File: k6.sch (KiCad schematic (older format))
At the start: 23 parts, among them J1 USB_C_Receptacle_USB2.0, J2 Conn_02x05_Odd_Even, SW1 SW_SPDT, SW2 SW_Push, U1 STM32F042K6T6, U2 MCP1700-3302E_SOT23

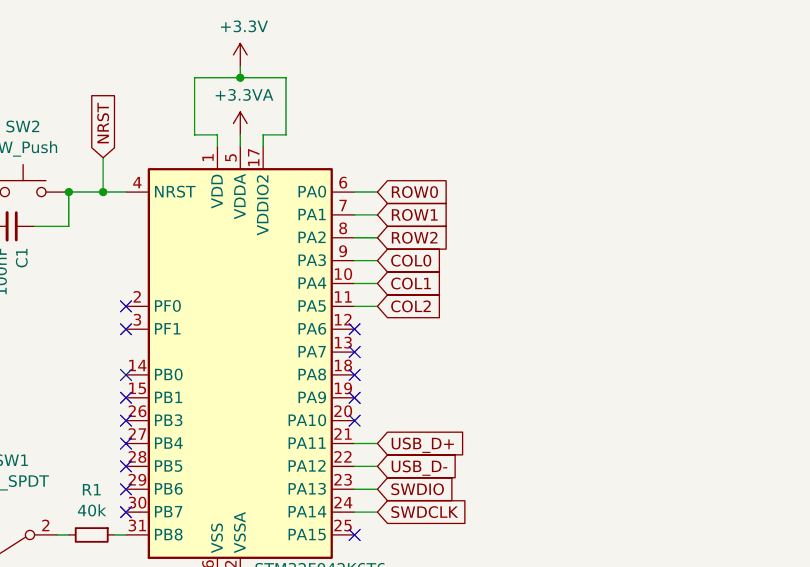
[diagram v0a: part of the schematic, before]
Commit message: Add some tracks - hate it
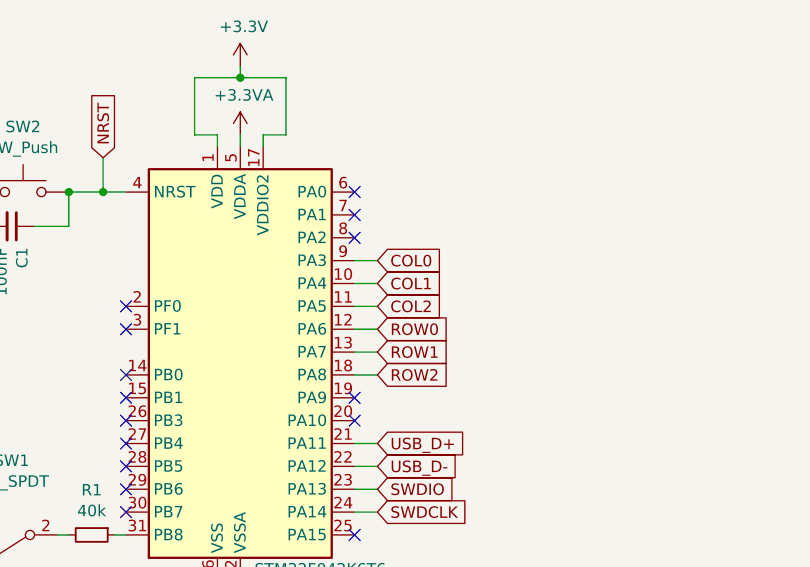
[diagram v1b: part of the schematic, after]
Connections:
- net ROW0: now also U1.12 (PA6); no longer U1.6 (PA0)
- net ROW1: now also U1.13 (PA7); no longer U1.7 (PA1)
- net ROW2: now also U1.18 (PA8); no longer U1.8 (PA2)
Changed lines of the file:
@@
 $EndDescr
-$Comp
-L MCU_ST_STM32F0:STM32F042K6Tx U1
-U 1 1 5EB61287
-P 2250 2550
-F 0 "U1" H 2350 1500 50  0000 C CNN
-F 1 "STM32F042K6T6" H 2600 1600 50  0000 C CNN
-F 2 "Package_QFP:LQFP-32_7x7mm_P0.8mm" H 1850 1650 50  0001 R CNN
-F 3 "http://www.st.com/st-web-ui/static/active/en/resource/technical/document/datasheet/DM00105814.pdf" H 2250 2550 50  0001 C CNN
-	1    2250 2550
-	1    0    0    -1
-$EndComp
 $Comp
 L Connector:USB_C_Receptacle_USB2.0 J1
@@
 $EndSheet
 Wire Wire Line
-	2150 3550 2250 3550
-Wire Wire Line
 	1850 3600 1850 3550
-Connection ~ 2150 3550
-Wire Wire Line
-	1850 3550 2150 3550
 $Comp
 L power:GND #PWR05
@@
 Wire Wire Line
 	1100 1850 1050 1850
-Text GLabel 2850 1850 2    50   Input ~ 0
+Text GLabel 2850 2450 2    50   Input ~ 0
 ROW0
-Text GLabel 2850 1950 2    50   Input ~ 0
+Text GLabel 2850 2550 2    50   Input ~ 0
 ROW1
-Text GLabel 2850 2050 2    50   Input ~ 0
+Text GLabel 2850 2650 2    50   Input ~ 0
 ROW2
 Text GLabel 2850 2150 2    50   Input ~ 0
@@
 COL2
 Wire Wire Line
-	2750 1850 2850 1850
-Wire Wire Line
-	2850 1950 2750 1950
-Wire Wire Line
-	2750 2050 2850 2050
-Wire Wire Line
 	2850 2150 2750 2150
 Wire Wire Line
@@
 Wire Wire Line
 	2850 2350 2750 2350
-NoConn ~ 2750 2450
-NoConn ~ 2750 2550
-NoConn ~ 2750 2650
 NoConn ~ 2750 2750
 NoConn ~ 2750 2850
@@
 $EndComp
 NoConn ~ 5600 3900
+Connection ~ 2150 3550
+Wire Wire Line
+	1850 3550 2150 3550
+Wire Wire Line
+	2150 3550 2250 3550
+$Comp
+L MCU_ST_STM32F0:STM32F042K6Tx U1
+U 1 1 5EB61287
+P 2250 2550
+F 0 "U1" H 2350 1500 50  0000 C CNN
+F 1 "STM32F042K6T6" H 2600 1600 50  0000 C CNN
+F 2 "Package_QFP:LQFP-32_7x7mm_P0.8mm" H 1850 1650 50  0001 R CNN
+F 3 "http://www.st.com/st-web-ui/static/active/en/resource/technical/document/datasheet/DM00105814.pdf" H 2250 2550 50  0001 C CNN
+	1    2250 2550
+	1    0    0    -1
+$EndComp
+Wire Wire Line
+	2750 2650 2850 2650
+Wire Wire Line
+	2850 2550 2750 2550
+Wire Wire Line
+	2750 2450 2850 2450
+NoConn ~ 2750 1850
+NoConn ~ 2750 1950
+NoConn ~ 2750 2050
 $EndSCHEMATC
